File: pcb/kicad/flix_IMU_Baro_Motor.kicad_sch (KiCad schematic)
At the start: 2 parts, among them IC2 BMP384, U2 ICM-40609-D

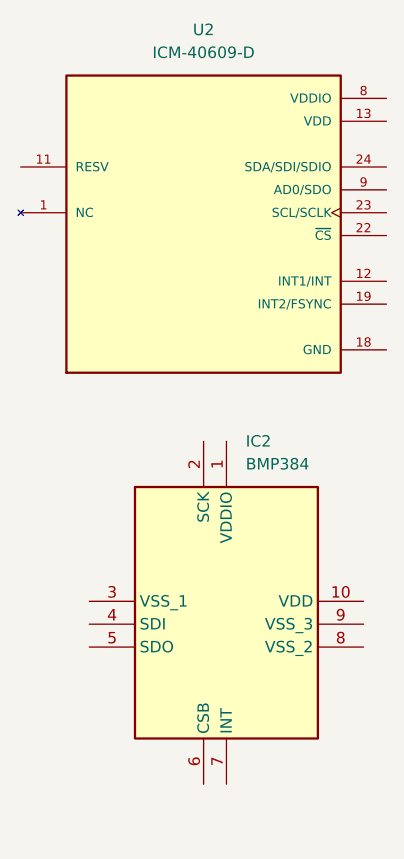
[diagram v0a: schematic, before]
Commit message: update sch structure
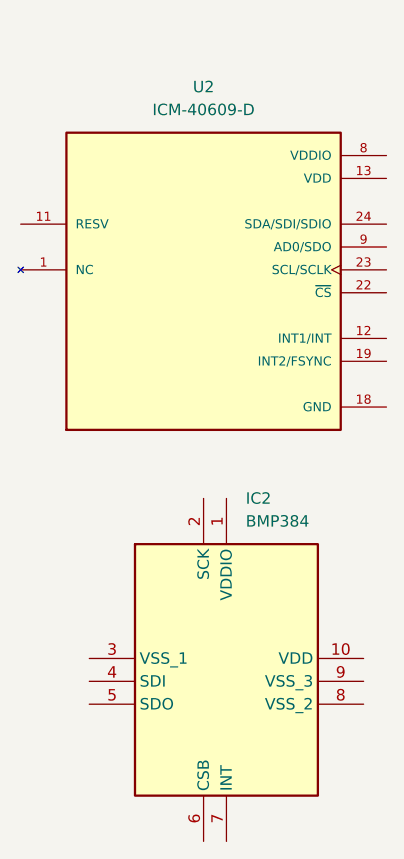
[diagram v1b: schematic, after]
